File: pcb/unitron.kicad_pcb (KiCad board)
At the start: 2 copper layers, 80.5 x 141 mm, 69 parts, among them J1 Conn_01x09_Female, J2 Conn_01x09_Male, J3 Conn_01x09_Female, J4 Conn_01x09_Male, J5 Conn_02x03_Odd_Even, Q1 FDN340P, Q2 BSS123, SW1 SW_SPST, U1 LTC-4727JS, U2 LTC-4727JS, U3 AS1115-BSST, U4 ATSAMD21E, U5 LTC-4727JR, U6 LTC-4727JR, U7 AS1115-BSST

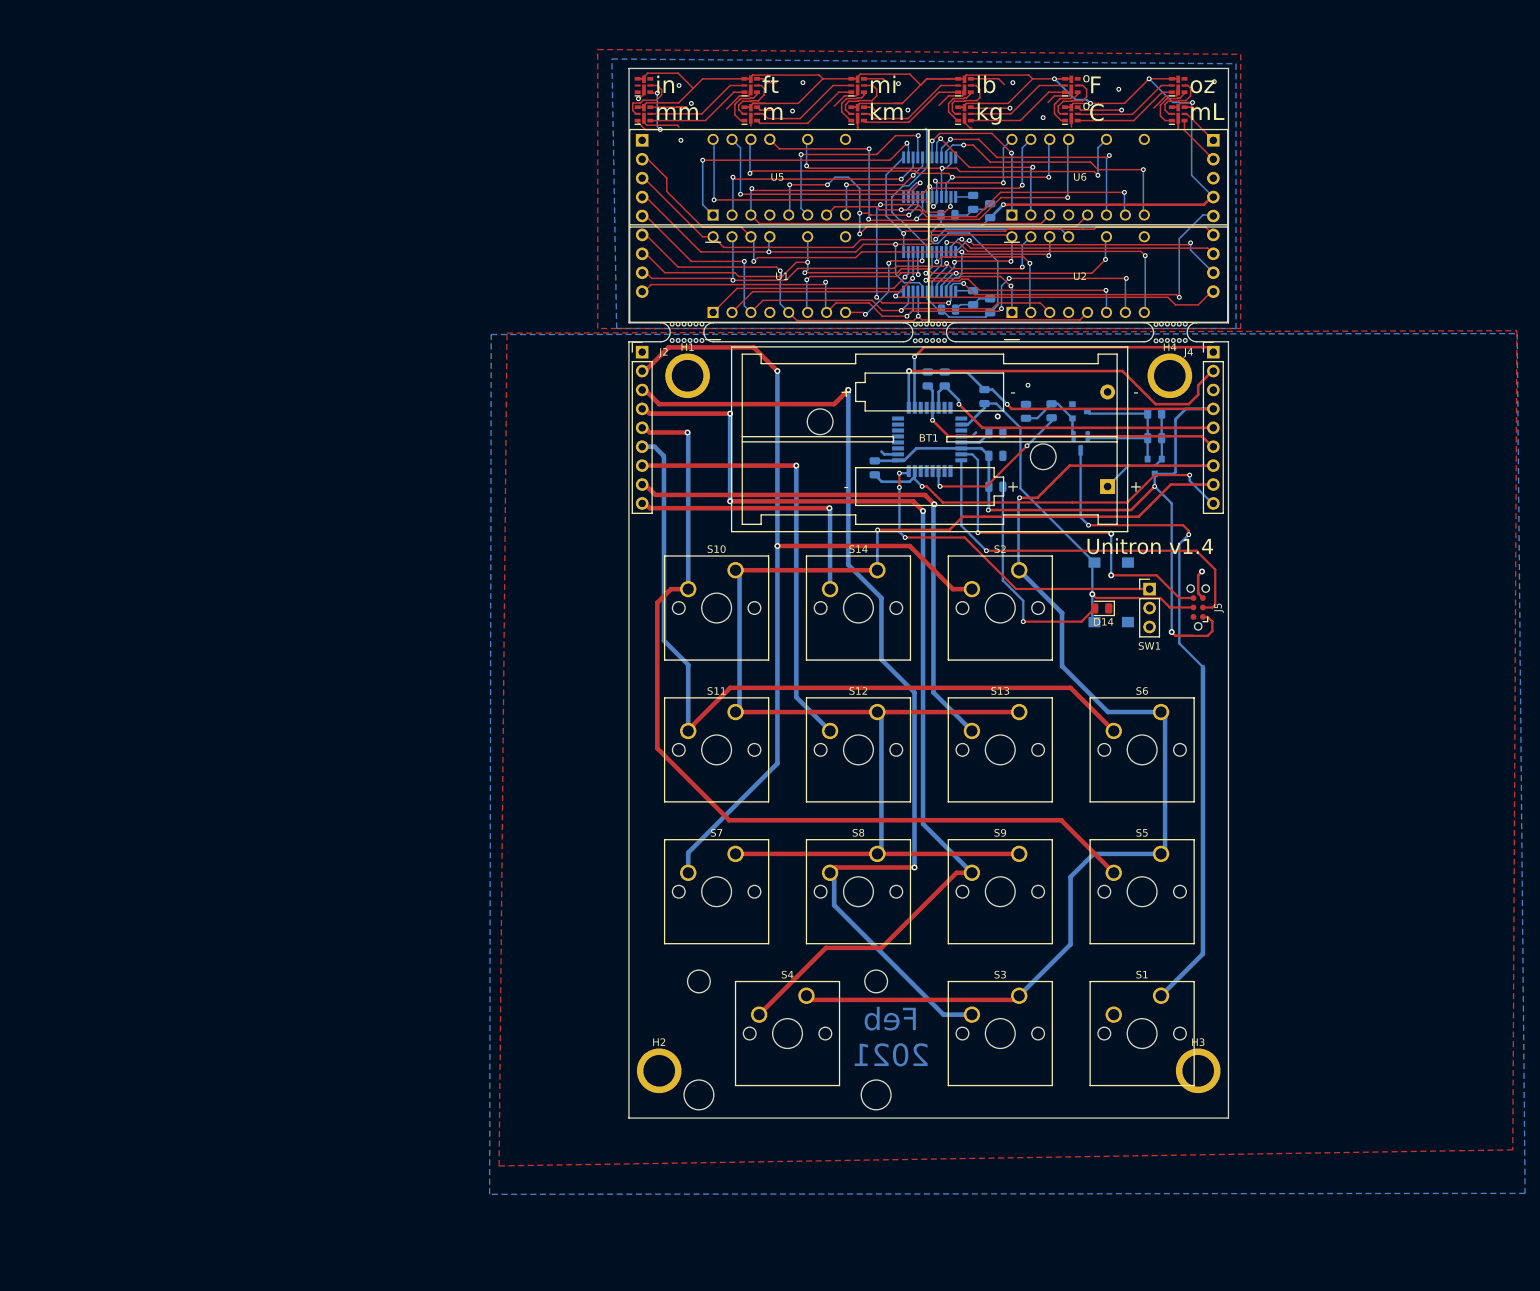
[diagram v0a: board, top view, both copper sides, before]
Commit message: PCB v1.5
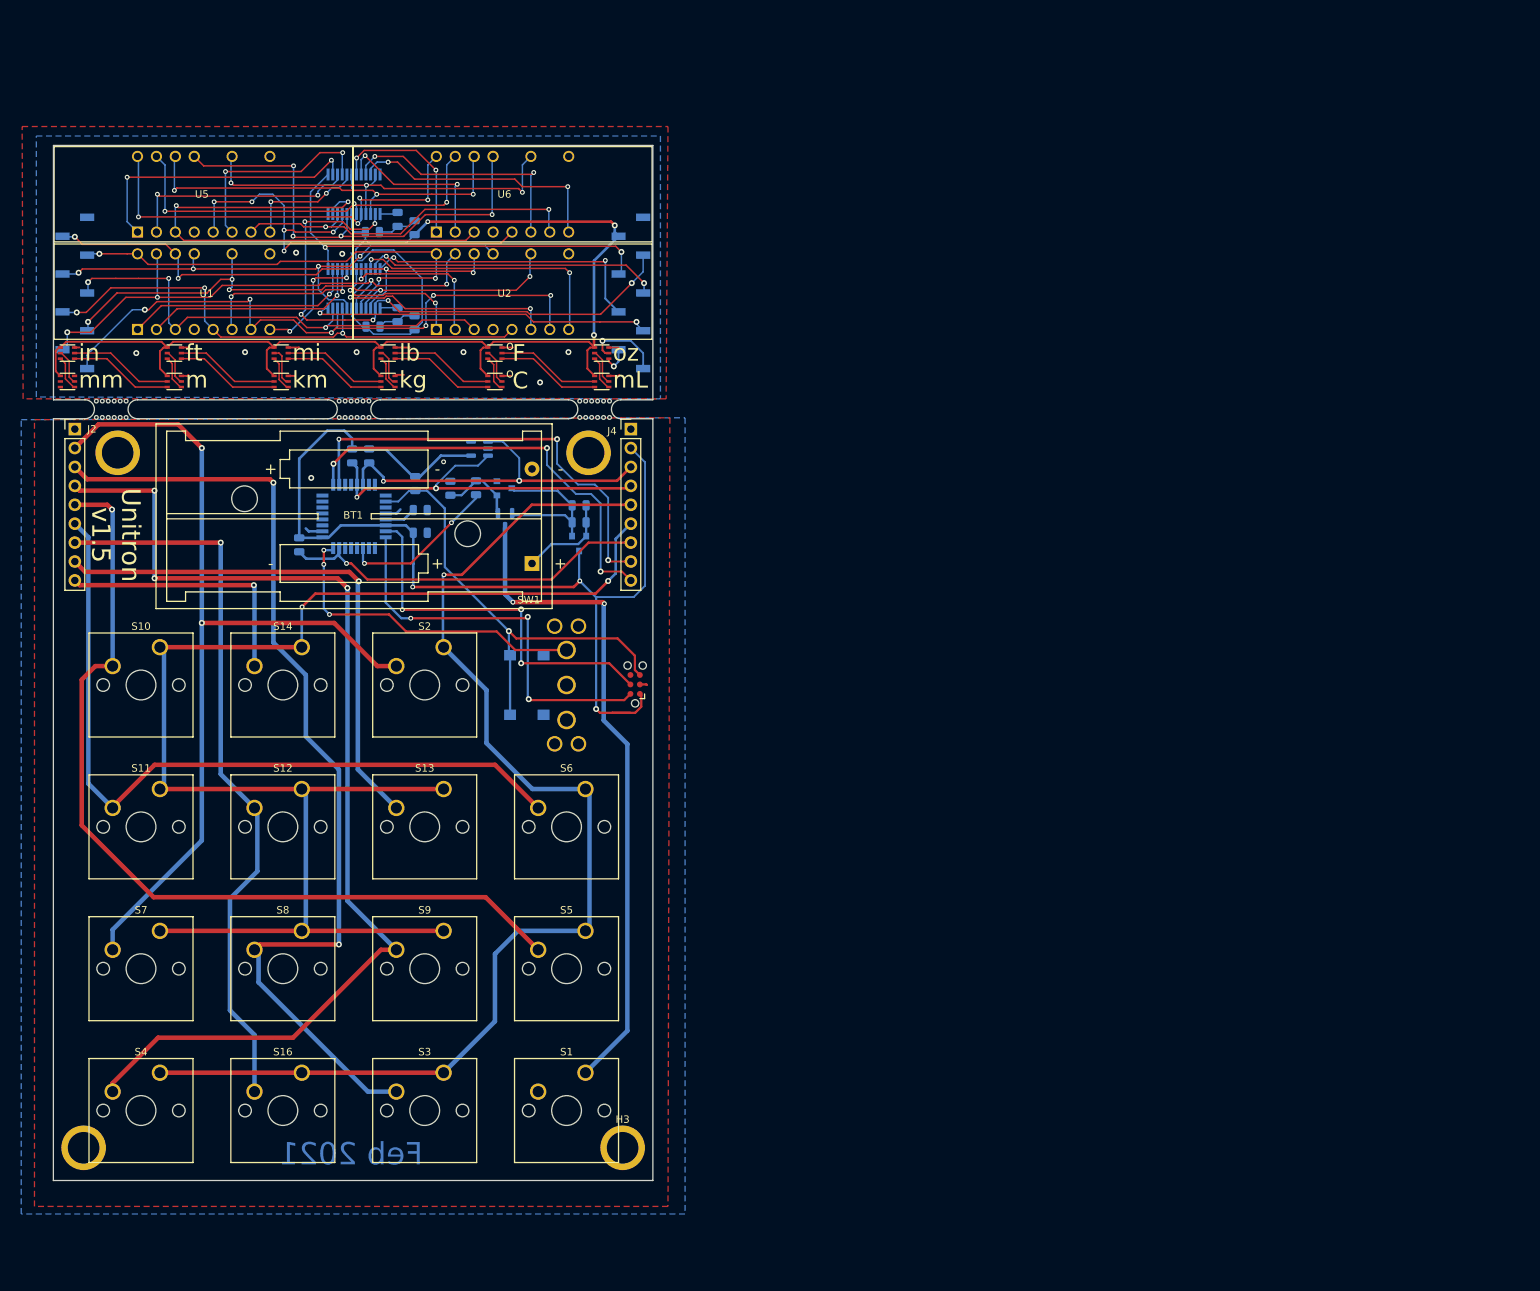
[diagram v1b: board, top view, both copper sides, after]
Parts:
- removed D14: LED, LED_SMD:LED_0805_2012Metric
- removed MB1, MB2, MB3: VAL**, asl_footprints:mouse-bite-2.54mm-slot-long
- removed R2: 10KΩ, Resistor_SMD:R_0805_2012Metric
- added MB*: VAL**, asl_footprints:mouse-bite-2.54mm-slot-long, F.Cu at (72.5, 66.1)
- added MB*: VAL**, asl_footprints:mouse-bite-2.54mm-slot-long, F.Cu at (105.1, 66.1)
- added MB*: VAL**, asl_footprints:mouse-bite-2.54mm-slot-long, F.Cu at (137.4, 66.1)
- added S16: Gateron Blue, Button_Switch_Keyboard:SW_Cherry_MX_1.00u_PCB, F.Cu at (98.0, 155.2)
- added U8: AT24C01C-STUM, Package_TO_SOT_SMD:SOT-23-5, B.Cu at (121.9, 71.4)
- BT1: value 2466 -> 2468
- D1, D10, D11, D12, D2, D3, D4, D5, D6, D7, D8, D9: footprint LED_SMD:LED-APA102-2020 -> asl_footprints:LED-APA102-2020
- J1, J3: footprint Connector_PinSocket_2.54mm:PinSocket_1x09_P2.54mm_Vertical -> Connector_PinSocket_2.54mm:PinSocket_1x09_P2.54mm_Vertical_SMD_Pin1Left
- S4: footprint Button_Switch_Keyboard:SW_Cherry_MX_2.00u_PCB -> Button_Switch_Keyboard:SW_Cherry_MX_1.00u_PCB
- SW1: footprint asl_footprints:B12AP -> asl_footprints:switch_nkk_reinforced_pc_pin
- moved S4 87.4 mm to (79.0, 155.2)
- moved D10 85.4 mm to (109.6, 62.4)
- moved D11 85.4 mm to (124.0, 62.4)
- moved D12 85.4 mm to (138.3, 62.4)
- moved D4 85.4 mm to (109.6, 58.5)
- moved D5 85.4 mm to (124.0, 58.5)
- moved D6 85.4 mm to (138.3, 58.5)
- moved D1 85.4 mm to (66.6, 58.5)
- moved D2 85.4 mm to (80.9, 58.5)
- moved D7 85.4 mm to (66.6, 62.4)
- moved D8 85.4 mm to (80.9, 62.4)
- moved D3 85.4 mm to (95.3, 58.5)
- moved D9 85.4 mm to (95.3, 62.4)
- moved J3 80.9 mm to (142.2, 50.5)
- moved S15 79.5 mm to (128.3, 103.1)
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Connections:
- BT1 pad 2: (no net) -> GND
- C2 pad 2: (no net) -> GND
- D1 pad 2: (no net) -> Net-(D1-Pad2)
- D1 pad 3: (no net) -> Net-(D1-Pad3)
- D12 pad 4: /SDI -> Net-(D12-Pad4)
- D12 pad 5: /CKI -> Net-(D12-Pad5)
- D3 pad 4: Net-(D3-Pad4) -> Net-(D10-Pad3)
- D3 pad 5: Net-(D3-Pad5) -> Net-(D10-Pad2)
- D4 pad 2: Net-(D4-Pad2) -> Net-(D10-Pad5)
- D4 pad 3: Net-(D4-Pad3) -> Net-(D10-Pad4)
- D4 pad 4: Net-(D10-Pad3) -> Net-(D11-Pad3)
- D4 pad 5: Net-(D10-Pad2) -> Net-(D11-Pad2)
- D5 pad 2: Net-(D10-Pad5) -> Net-(D11-Pad5)
- D5 pad 3: Net-(D10-Pad4) -> Net-(D11-Pad4)
- D5 pad 4: Net-(D11-Pad3) -> Net-(D12-Pad3)
- D5 pad 5: Net-(D11-Pad2) -> Net-(D12-Pad2)
- D6 pad 2: Net-(D11-Pad5) -> Net-(D12-Pad5)
- D6 pad 3: Net-(D11-Pad4) -> Net-(D12-Pad4)
- D6 pad 4: Net-(D12-Pad3) -> /CKI
- D6 pad 5: Net-(D12-Pad2) -> /SDI
- D7 pad 2: Net-(D1-Pad5) -> (no net)
- D7 pad 3: Net-(D1-Pad4) -> (no net)
- D7 pad 4: Net-(D2-Pad3) -> Net-(D1-Pad3)
- D7 pad 5: Net-(D2-Pad2) -> Net-(D1-Pad2)
- D8 pad 2: Net-(D2-Pad5) -> Net-(D1-Pad5)
- D8 pad 3: Net-(D2-Pad4) -> Net-(D1-Pad4)
- D8 pad 4: Net-(D3-Pad3) -> Net-(D2-Pad3)
- D8 pad 5: Net-(D3-Pad2) -> Net-(D2-Pad2)
- D9 pad 2: Net-(D3-Pad5) -> Net-(D2-Pad5)
- D9 pad 3: Net-(D3-Pad4) -> Net-(D2-Pad4)
- D9 pad 4: Net-(D4-Pad3) -> Net-(D3-Pad3)
- D9 pad 5: Net-(D4-Pad2) -> Net-(D3-Pad2)
- J3 pad 1: /CKI -> /GND_daughter
- J3 pad 2: /SDI -> /VIN_daughter
- J3 pad 3: /GND_daughter -> /SCL
- J3 pad 4: /VIN_daughter -> /SDA
- J3 pad 5: /SCL -> Net-(J3-Pad5)
- J3 pad 6: /SDA -> Net-(J3-Pad6)
- J3 pad 7: Net-(J3-Pad7) -> /IRQ
- J3 pad 8: Net-(J3-Pad8) -> /CKI
- J3 pad 9: /IRQ -> /SDI
- J4 pad 1: /SCK -> GND
- J4 pad 2: /MOSI -> /VIN
- J4 pad 3: GND -> /SCL_mcu
- J4 pad 4: /VIN -> /SDA_mcu
- J4 pad 5: /SCL_mcu -> /KEYA
- J4 pad 6: /SDA_mcu -> /KEYB
- J4 pad 7: /KEYA -> /IRQ_mcu
- J4 pad 8: /KEYB -> /SCK
- J4 pad 9: /IRQ_mcu -> /MOSI
- U3 pad 11: Net-(J3-Pad7) -> Net-(J3-Pad5)
- U3 pad 12: Net-(J3-Pad8) -> Net-(J3-Pad6)
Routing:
- net /GND_daughter: track 92.4 -> 18.6 mm, vias 14 -> 8
- net Net-(J2-Pad7): track 57.8 -> 98.3 mm
- net Net-(J3-Pad5): track 0.00 -> 40.1 mm, vias 0 -> 2
- net Net-(J3-Pad6): track 0.00 -> 38.8 mm, vias 0 -> 2
- net /VIN_daughter: track 232.5 -> 194.7 mm, vias 5 -> 3
- net Net-(J3-Pad8): track 37.6 -> 0.00 mm, vias 2 -> 0
- net Net-(J3-Pad7): track 37.0 -> 0.00 mm, vias 1 -> 0
- net Net-(D14-Pad2): track 29.6 -> 0.00 mm, vias 1 -> 0
- net Net-(D4-Pad2): track 14.8 -> 0.00 mm
- net Net-(D4-Pad3): track 14.4 -> 0.00 mm
- net /SCK: track 47.8 -> 59.0 mm, vias 1 -> 3
- net /KEYA: track 149.4 -> 160.5 mm
- net Net-(D3-Pad3): track 14.5 -> 4.73 mm
- net Net-(D3-Pad2): track 14.8 -> 5.19 mm
- net Net-(D10-Pad4): track 14.2 -> 4.68 mm
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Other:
- board size 80.5 x 141 mm -> 80.5 x 139 mm
- board text added: "Unitron v1.5"
- board text removed: "Unitron v1.4"

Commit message: pcb v1.6
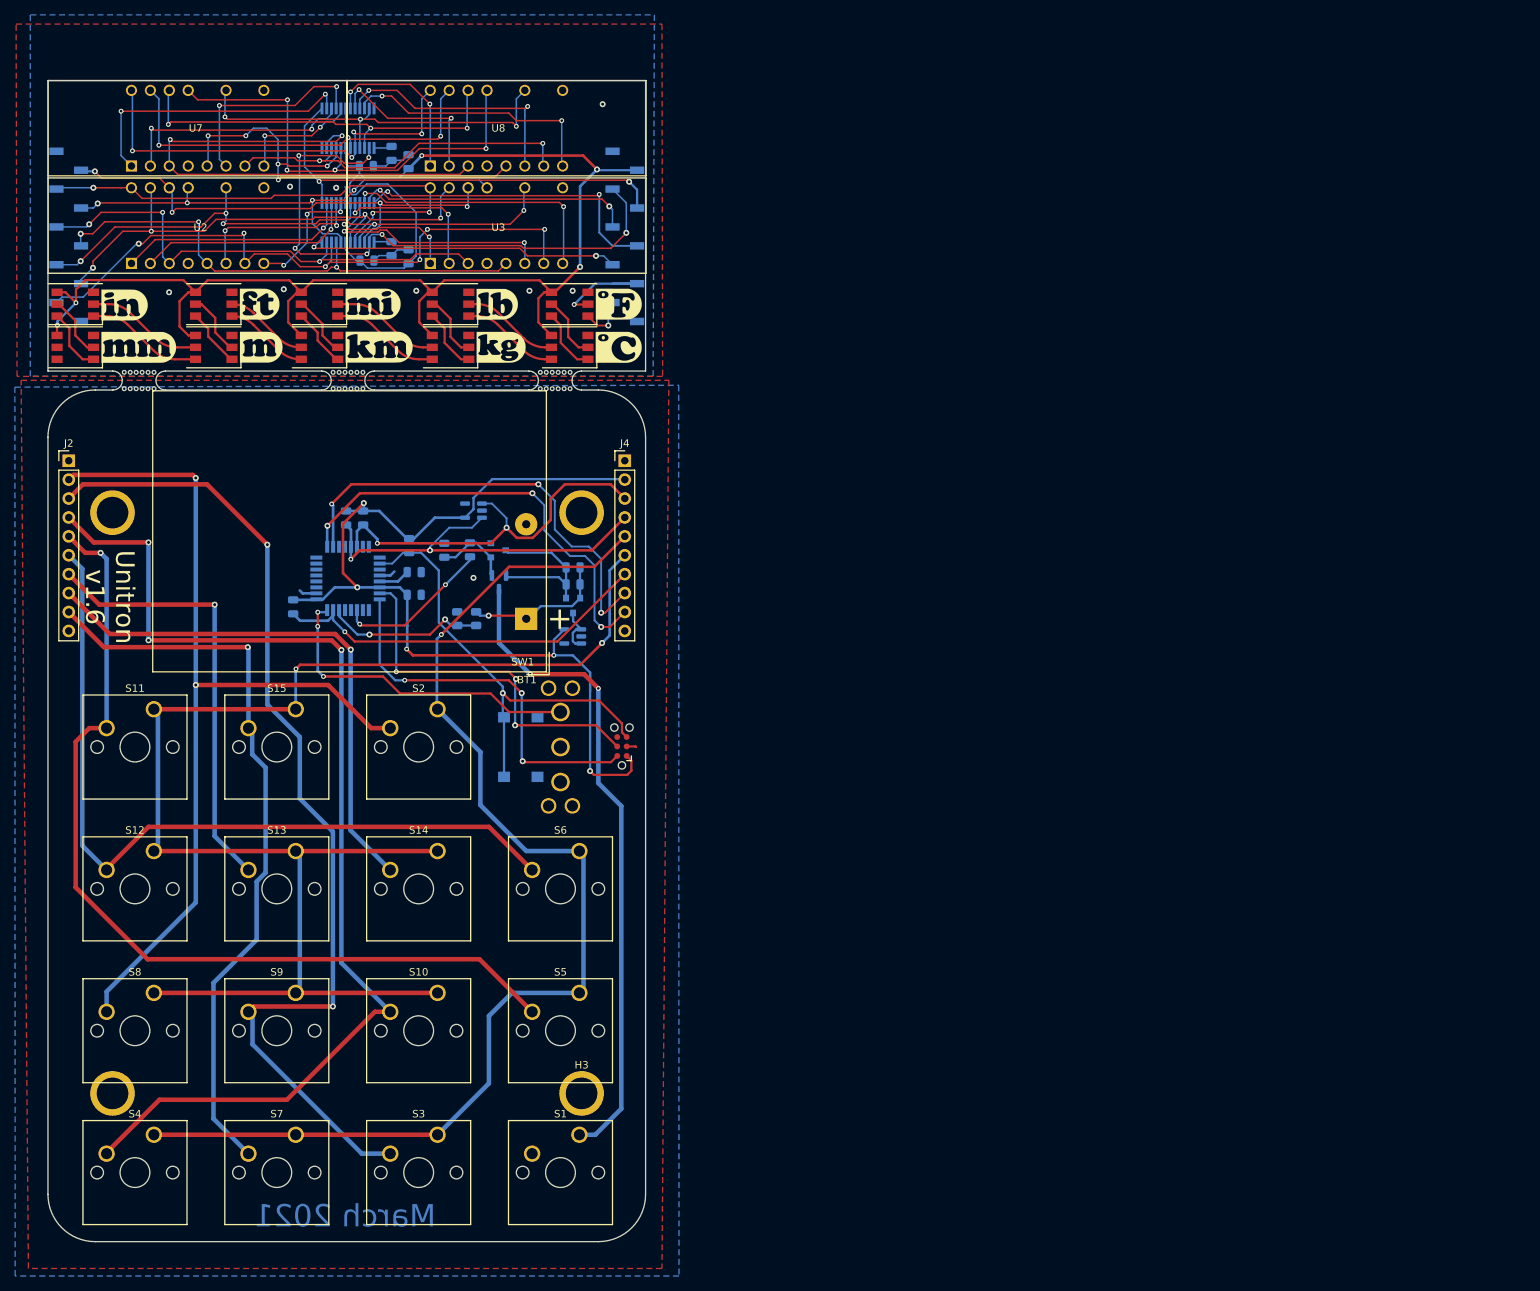
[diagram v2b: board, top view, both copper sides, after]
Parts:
- removed the D11 at (124.0, 62.4)
- removed D12: APA102-2020, asl_footprints:LED-APA102-2020
- added G***: LOGO, LOGO, F.Cu at (89.7, 52.0)
- added G***: LOGO, LOGO, F.Cu at (137.5, 57.8)
- added G***: LOGO, LOGO, F.Cu at (121.5, 57.8)
- added G***: LOGO, LOGO, F.Cu at (103.9, 57.8)
- added G***: LOGO, LOGO, F.Cu at (89.7, 57.8)
- added G***: LOGO, LOGO, F.Cu at (71.1, 52.1)
- added G***: LOGO, LOGO, F.Cu at (71.1, 57.8)
- added G***: LOGO, LOGO, F.Cu at (137.5, 52.0)
- added G***: LOGO, LOGO, F.Cu at (103.9, 52.0)
- added G***: LOGO, LOGO, F.Cu at (121.5, 52.0)
- added R7: 10KΩ, Resistor_SMD:R_0805_2012Metric, B.Cu at (121.5, 94.2)
- added R8: 10KΩ, Resistor_SMD:R_0805_2012Metric, B.Cu at (118.9, 94.2)
- added U1: AP2112K-3.3, Package_TO_SOT_SMD:SOT-23-5, B.Cu at (134.4, 96.6)
- BT1: footprint Battery:BatteryHolder_Keystone_2468_2xAAA -> Battery:BatteryHolder_Keystone_2479_3xAAA
- C2, C3: value 0.1µF -> 100nF
- D1, D10, D2, D3, D4, D5, D6, D7, D8, D9: value APA102-2020 -> SK9822; footprint asl_footprints:LED-APA102-2020 -> asl_footprints:LED_SK9822_5050
- J1, J3: value Conn_01x09_Female -> Conn_01x10_Male; footprint Connector_PinSocket_2.54mm:PinSocket_1x09_P2.54mm_Vertical_SMD_Pin1Left -> Connector_PinSocket_2.54mm:PinSocket_1x10_P2.54mm_Vertical_SMD_Pin1Right
- J2, J4: value Conn_01x09_Male -> Conn_01x10_Female; footprint Connector_PinHeader_2.54mm:PinHeader_1x09_P2.54mm_Vertical -> Connector_PinHeader_2.54mm:PinHeader_1x10_P2.54mm_Vertical
- moved D6 70.7 mm to (67.6, 57.8), turned to 180 degrees
- moved BT1 26.9 mm to (128.2, 94.2)
- moved D10 24.8 mm to (134.0, 57.8), turned to 180 degrees
- moved D9 23.2 mm to (118.0, 57.8), turned to 180 degrees
- moved D7 20.2 mm to (86.2, 57.8), turned to 180 degrees
- moved D8 20.0 mm to (100.4, 57.8), turned to 180 degrees
- moved D5 12.0 mm to (134.0, 52.0), turned to 180 degrees
- moved D4 10.7 mm to (118.0, 52.0), turned to 180 degrees
- moved H3 9.15 mm to (135.6, 158.0)
- moved U3 8.91 mm to (124.2, 41.4)
- moved U8 8.91 mm to (124.2, 28.3)
- moved R13 8.91 mm to (106.7, 33.4)
- moved R4 8.91 mm to (112.4, 45.6)
- moved R5 8.91 mm to (106.8, 46.1)
- moved R6 8.91 mm to (110.1, 44.5)
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- renumbered D13 to D11, R9 to R10, R10 to R11, R11 to R12, R12 to R13, R13 to R14, R14 to R15, R3 to R2, R4 to R3, R5 to R4, R6 to R5, R7 to R6, R8 to R9, S9 to S10, S10 to S11, S11 to S12, S12 to S13, S13 to S14, S14 to S15, S15 to S16, S16 to S7, S7 to S8, S8 to S9, U1 to U2, U2 to U3, U3 to U4, U4 to U5, U8 to U6, U5 to U7, U6 to U8, U7 to U9
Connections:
- D1 pad 1: /VIN_daughter -> Net-(D1-Pad1)
- D1 pad 3: Net-(D1-Pad3) -> /GND_daughter
- D1 pad 4: Net-(D1-Pad4) -> /VIN_daughter
- D1 pad 6: /GND_daughter -> Net-(D1-Pad6)
- D10 pad 1: /VIN_daughter -> Net-(D10-Pad1)
- D10 pad 3: Net-(D10-Pad3) -> /GND_daughter
- D10 pad 4: Net-(D10-Pad4) -> /VIN_daughter
- D10 pad 6: /GND_daughter -> Net-(D10-Pad6)
- D2 pad 1: /VIN_daughter -> Net-(D2-Pad1)
- D2 pad 3: Net-(D2-Pad3) -> /GND_daughter
- D2 pad 4: Net-(D2-Pad4) -> /VIN_daughter
- D2 pad 6: /GND_daughter -> Net-(D2-Pad6)
- D3 pad 1: /VIN_daughter -> Net-(D3-Pad1)
- D3 pad 3: Net-(D3-Pad3) -> /GND_daughter
- D3 pad 4: Net-(D10-Pad3) -> /VIN_daughter
- D3 pad 5: Net-(D10-Pad2) -> Net-(D3-Pad5)
- D3 pad 6: /GND_daughter -> Net-(D3-Pad6)
- D4 pad 1: /VIN_daughter -> Net-(D10-Pad6)
- D4 pad 3: Net-(D10-Pad4) -> /GND_daughter
- D4 pad 4: Net-(D11-Pad3) (its old number) -> /VIN_daughter
- D4 pad 5: Net-(D11-Pad2) -> Net-(D4-Pad5)
- D4 pad 6: /GND_daughter -> Net-(D4-Pad6)
- D5 pad 1: /VIN_daughter -> /SDI
- D5 pad 2: Net-(D11-Pad5) -> /CKI
- D5 pad 3: Net-(D11-Pad4) -> /GND_daughter
- D5 pad 4: Net-(D12-Pad3) -> /VIN_daughter
- D5 pad 5: Net-(D12-Pad2) -> Net-(D10-Pad2)
- D5 pad 6: /GND_daughter -> Net-(D10-Pad1)
- D6 pad 1: /VIN_daughter -> Net-(D1-Pad6)
- D6 pad 2: Net-(D12-Pad5) -> Net-(D1-Pad5)
- D6 pad 3: Net-(D12-Pad4) -> /GND_daughter
- D6 pad 4: /CKI -> /VIN_daughter
- D6 pad 5: /SDI -> (no net)
- D6 pad 6: /GND_daughter -> (no net)
- D7 pad 1: /VIN_daughter -> Net-(D2-Pad6)
- D7 pad 2: (no net) -> Net-(D2-Pad5)
- D7 pad 3: (no net) -> /GND_daughter
- D7 pad 4: Net-(D1-Pad3) -> /VIN_daughter
- D7 pad 6: /GND_daughter -> Net-(D1-Pad1)
- D8 pad 1: /VIN_daughter -> Net-(D3-Pad6)
- D8 pad 2: Net-(D1-Pad5) -> Net-(D3-Pad5)
- D8 pad 3: Net-(D1-Pad4) -> /GND_daughter
- D8 pad 4: Net-(D2-Pad3) -> /VIN_daughter
- D8 pad 6: /GND_daughter -> Net-(D2-Pad1)
- D9 pad 1: /VIN_daughter -> Net-(D4-Pad6)
- D9 pad 2: Net-(D2-Pad5) -> Net-(D4-Pad5)
- D9 pad 3: Net-(D2-Pad4) -> /GND_daughter
- D9 pad 4: Net-(D3-Pad3) -> /VIN_daughter
- D9 pad 6: /GND_daughter -> Net-(D3-Pad1)
- Q1 pad 3: /VIN -> Net-(Q1-Pad3)
- S7 pad 2: Net-(J2-Pad7) -> Net-(J2-Pad9)
- U5 pad 6: (no net) -> /batt_lvl
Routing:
- net Net-(J2-Pad9): track 35.2 -> 99.9 mm
- net Net-(J2-Pad7): track 98.3 -> 59.3 mm
- net /batt_lvl: track 0.00 -> 21.8 mm, vias 0 -> 2
- net Net-(D1-Pad1): track 0.00 -> 15.7 mm
- net Net-(D3-Pad1): track 0.00 -> 14.7 mm
- net Net-(D11-Pad3) (its old number): track 14.0 -> 0.00 mm
- net Net-(D2-Pad4): track 14.0 -> 0.00 mm
- net Net-(D12-Pad3): track 14.0 -> 0.00 mm
- net Net-(D12-Pad2): track 14.0 -> 0.00 mm
- net Net-(D11-Pad2): track 14.0 -> 0.00 mm
- net Net-(D10-Pad3): track 14.0 -> 0.00 mm
- net Net-(D1-Pad4): track 14.0 -> 0.00 mm
- net /GND_daughter: track 18.6 -> 4.85 mm
- net Net-(D10-Pad6): track 0.00 -> 13.1 mm
- net /VIN_daughter: track 194.7 -> 207.2 mm, vias 3 -> 5
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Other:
- board size 80.5 x 139 mm -> 80.3 x 155.9 mm
- board text added: "March 2021"
- board text added: "Unitron v1.6"
- board text removed: "C"
- board text removed: "F"
- board text removed: "Feb 2021"
- board text removed: "Unitron v1.5"
- board text removed: "ft m"
- board text removed: "in mm"
- board text removed: "lb kg"
- board text removed: "mi km"
- board text removed: "o"
- board text removed: "oz mL"
